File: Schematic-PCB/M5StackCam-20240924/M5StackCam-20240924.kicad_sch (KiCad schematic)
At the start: 3 parts, among them J1 Conn_CamL, J2 Conn_CamR, J3 Conn_Main

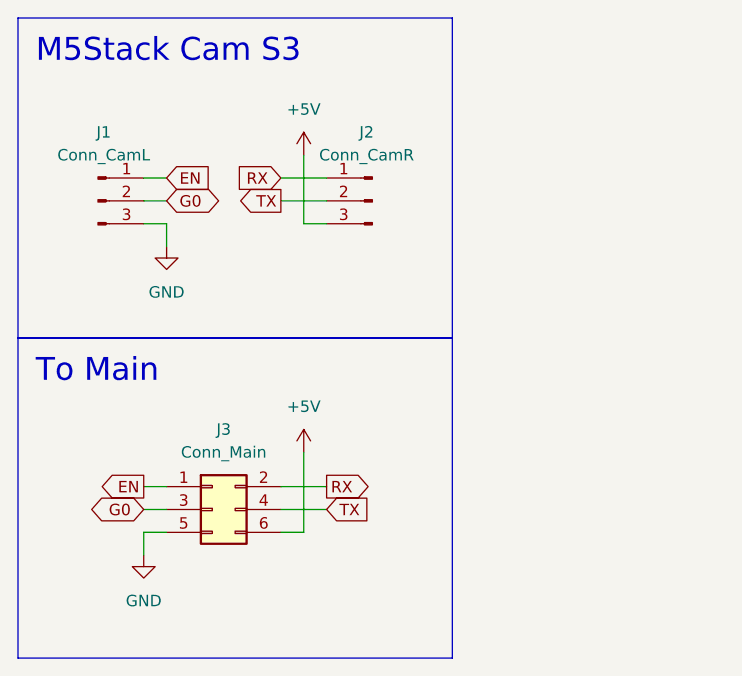
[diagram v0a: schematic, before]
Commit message: update: カメラ用基板を更新した
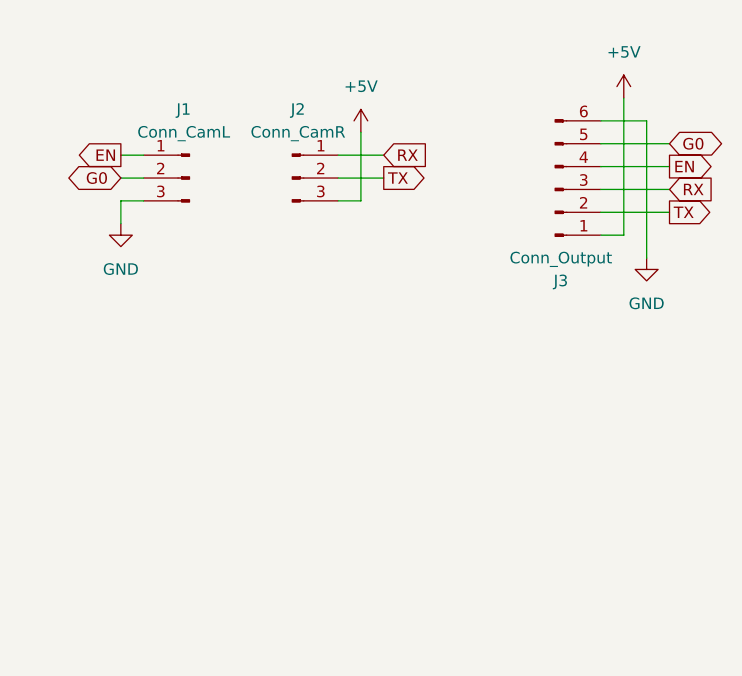
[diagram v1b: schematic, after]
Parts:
- removed J3: Conn_Main, Connector_PinHeader_2.54mm:PinHeader_2x03_P2.54mm_Vertical, symbol Connector_Generic:Conn_02x03_Odd_Even
- added J3: Conn_Output, Connector_PinHeader_2.54mm:PinHeader_1x06_P2.54mm_Horizontal, symbol Connector:Conn_01x06_Pin
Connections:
- net +5V: now also J3.1 (Pin_1)
- net EN: now also J3.4 (Pin_4)
- net G0: now also J3.5 (Pin_5)
- net GND: now also J3.6 (Pin_6)
- net RX: now also J3.3 (Pin_3)
- net TX: now also J3.2 (Pin_2)
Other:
- moved on the sheet: J2
